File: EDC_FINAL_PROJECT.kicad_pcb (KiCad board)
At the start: 2 copper layers, 88.9 x 50.8 mm, 31 parts, among them J1 Screw_Terminal_01x02, J2 Screw_Terminal_01x03, SW1 SW_Push_DPDT, U1 LM317_TO-220, U2 LM337_TO220

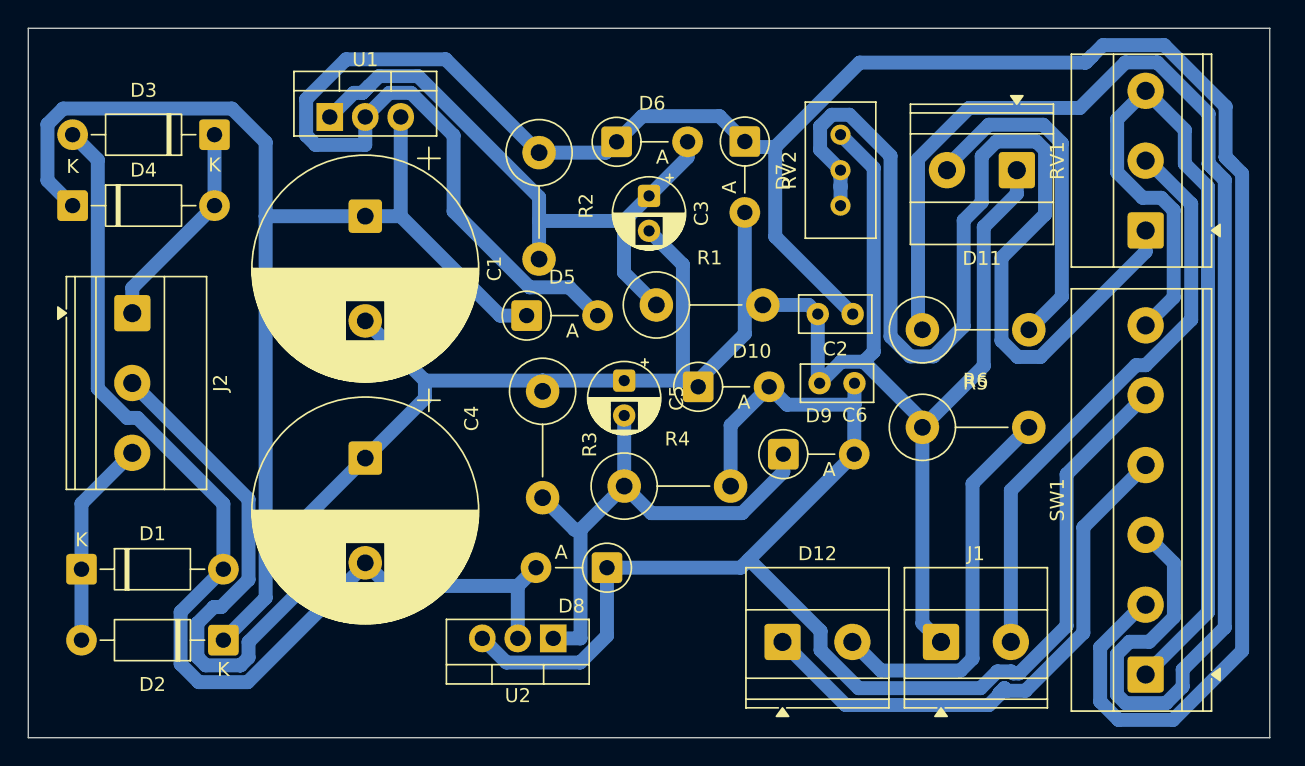
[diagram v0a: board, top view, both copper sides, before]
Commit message: 10.12.2025 --final revision
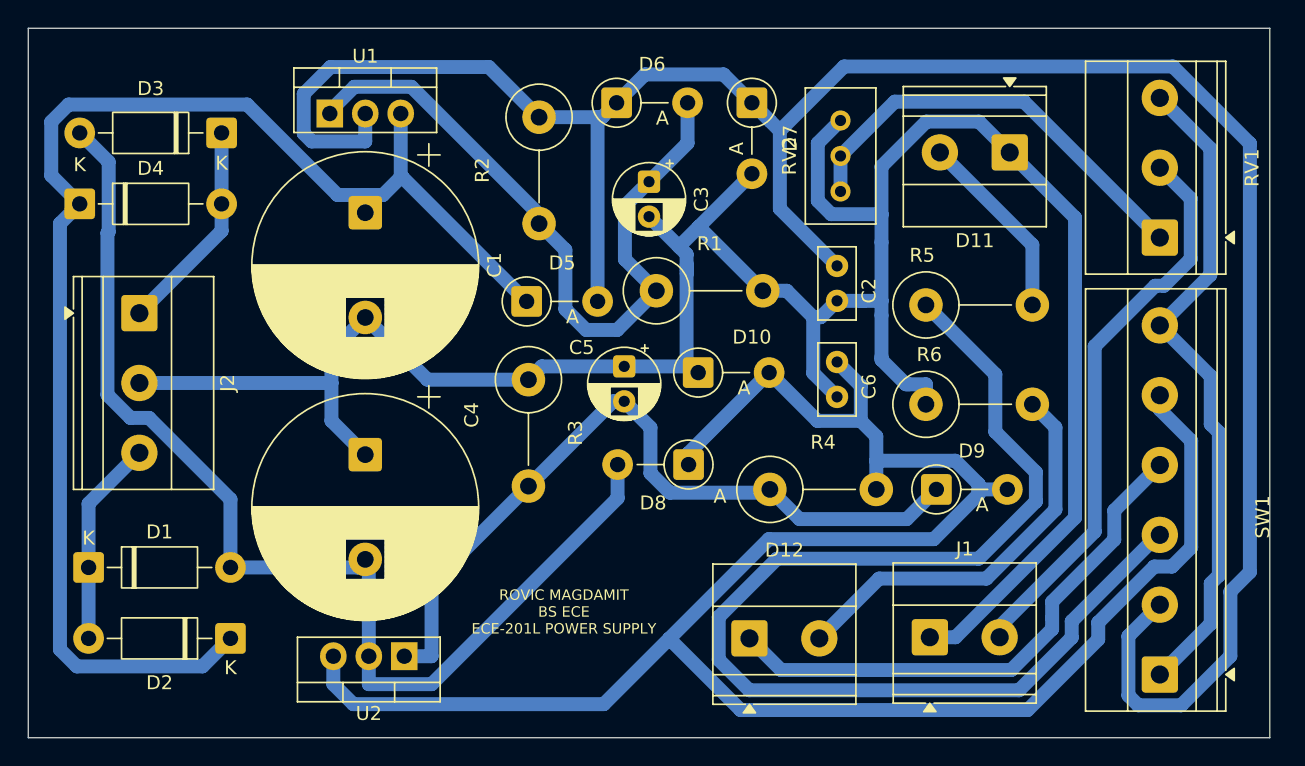
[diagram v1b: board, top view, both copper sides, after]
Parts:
- moved D9 11.2 mm to (132.1, 105.2)
- moved U2 10.7 mm to (94.0, 117.1)
- moved R4 10.4 mm to (120.2, 105.2)
- moved D8 9.41 mm to (114.3, 103.4)
- moved C2 3.62 mm to (125.0, 89.2), turned to -90 degrees
- moved D7 2.82 mm to (118.9, 77.5)
- moved D6 2.79 mm to (109.2, 77.5)
- moved R2 2.54 mm to (103.6, 78.5)
- moved D12 2.38 mm to (118.7, 115.8)
- moved R5 1.80 mm to (131.3, 91.9)
- moved R6 1.67 mm to (131.3, 99.1)
- moved C6 1.59 mm to (125.0, 98.5), turned to 90 degrees
- moved D11 1.37 mm to (137.3, 81.0)
- moved R3 1.31 mm to (102.9, 97.3)
- moved RV1 1.14 mm to (148.1, 87.1)
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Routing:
- net Net-(RV1-Pad1): track 80.9 -> 31.0 mm
- net Net-(D10-A): track 104.5 -> 149.9 mm
- net Net-(D5-A): track 189.1 -> 165.0 mm
- net Net-(RV1-Pad3): track 66.4 -> 47.8 mm
- net Net-(D9-K): track 37.6 -> 55.2 mm
- net Net-(R5-Pad1): track 101.2 -> 84.3 mm
- net Net-(D11-A): track 24.6 -> 13.7 mm
- net Net-(D2-K): track 89.3 -> 100.0 mm
- net Net-(D6-A): track 45.5 -> 51.8 mm
- net Net-(D10-K): track 181.5 -> 177.8 mm
- net Net-(D1-A): track 78.7 -> 81.1 mm
- net Net-(J1-Pin_2): track 41.7 -> 40.6 mm
- net Net-(D12-A): track 28.0 -> 29.0 mm
- net Net-(D12-K): track 39.6 -> 38.8 mm
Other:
- board text added: "ROVIC MAGDAMIT BS ECE ECE-201L POWER SUPPLY"
